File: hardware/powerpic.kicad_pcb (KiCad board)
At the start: 2 copper layers, 25.6 x 27.6 mm, 17 parts, among them U1 PIC16LF1919x-I/MR, Y1 32.768kHz

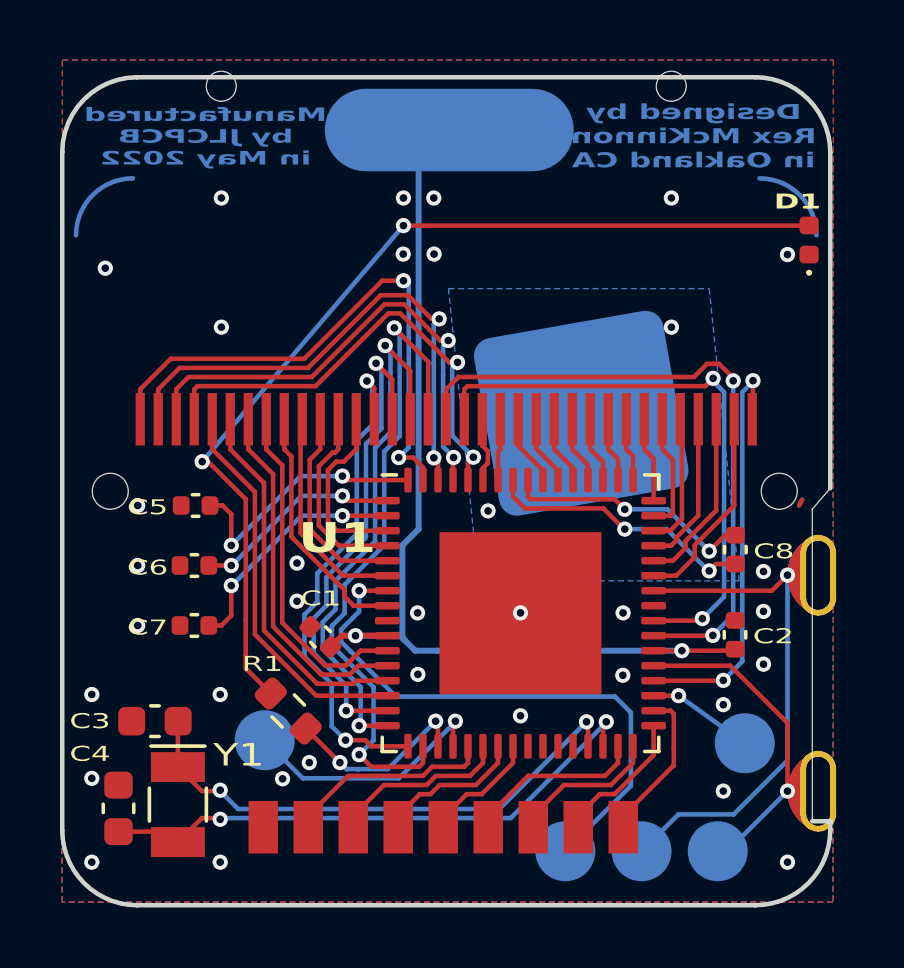
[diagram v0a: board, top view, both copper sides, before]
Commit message: release version 2.1
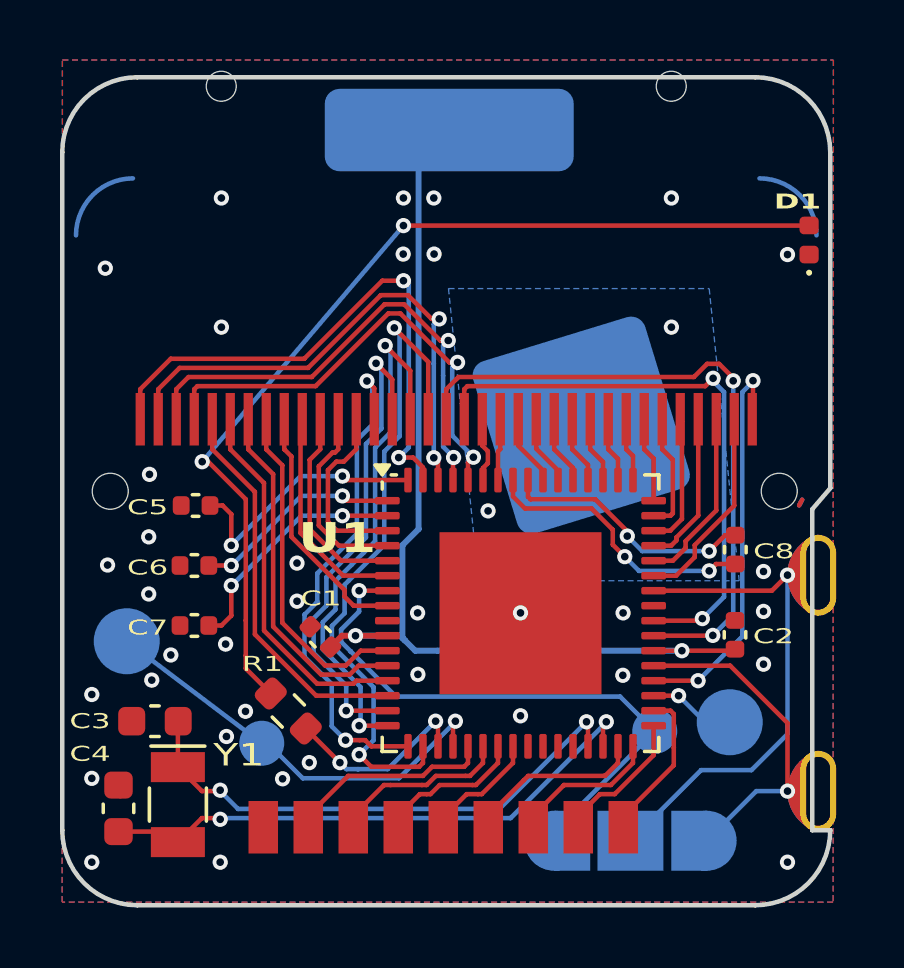
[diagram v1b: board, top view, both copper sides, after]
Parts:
- removed TP1: ~{MCLR}, powerpic:Progo_Pad_D2.0mm
- removed TP2: Mode, powerpic:Progo_Pad_D2.0mm
- removed TP3: Adj, powerpic:Progo_Pad_D2.0mm
- removed TP4: Debug, powerpic:Progo_Pad_D2.0mm
- added kibuzzard-6619F1C8: G***, kibuzzard-6619F1C8, B.Cu at (134.2, 67.7)
- added kibuzzard-6619F370: G***, kibuzzard-6619F370, B.Cu at (140.3, 61.6)
- added kibuzzard-6619F3FA: G***, kibuzzard-6619F3FA, B.Cu at (136.2, 64.0)
- added kibuzzard-6619F45C: G***, kibuzzard-6619F45C, B.Cu at (122.3, 62.6)
- added kibuzzard-6619F682: G***, kibuzzard-6619F682, B.Cu at (133.9, 49.7)
- added kibuzzard-6619F6E4: G***, kibuzzard-6619F6E4, B.Cu at (131.0, 46.7)
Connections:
- U1 pad 25: /RH1 -> unconnected-(U1-COM5/RH1-Pad25)
- U1 pad 26: /RH0 -> unconnected-(U1-COM4/RH0-Pad26)
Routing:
- net /BUZZ: track 8.55 -> 14.2 mm
- net /DEBUG: track 3.55 -> 2.90 mm
- net /~{MCLR}: track 19.1 -> 19.6 mm
- net GND: vias 35 -> 38
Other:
- outline, holes or cut-outs redrawn
- board text added: "2416"
- board text added: "REXCM"
- board text added: "v2.1"
- board text removed: "2.0"
- board text removed: "BUZ"
- board text removed: "DBG"
- board text removed: "Designed by Rex McKinnon in Oakland CA"
- board text removed: "GND"
- board text removed: "ICSP"
- board text removed: "Manufactured by JLCPCB in May 2022"
- board text removed: "VIN"
